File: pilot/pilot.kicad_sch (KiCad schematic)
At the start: 0 parts

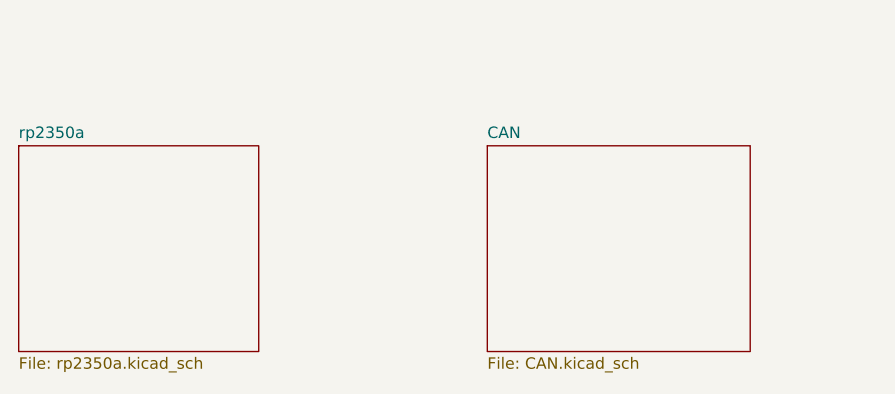
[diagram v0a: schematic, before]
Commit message: 2025/12/05/1722
初めてのコミット
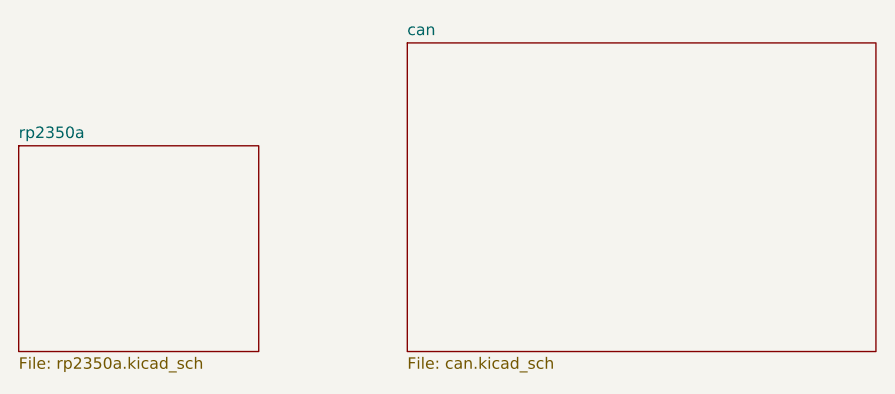
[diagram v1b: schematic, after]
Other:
- removed sheet CAN
- added sheet can (can.kicad_sch)
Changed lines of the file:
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@@
 	(paper "A4")
 	(sheet
-		(at 180.34 90.17)
-		(size 29.21 22.86)
+		(at 171.45 78.74)
+		(size 52.07 34.29)
 		(exclude_from_sim no)
 		(in_bom yes)
@@
 			(color 0 0 0 0.0000)
 		)
-		(property "Sheetname" "CAN"
-			(at 180.34 89.4584 0)
+		(property "Sheetname" "can"
+			(at 171.45 78.0284 0)
 			(effects
 				(font
@@
 			)
 		)
-		(property "Sheetfile" "CAN.kicad_sch"
-			(at 180.34 113.6146 0)
+		(property "Sheetfile" "can.kicad_sch"
+			(at 171.45 113.6146 0)
 			(effects
 				(font
